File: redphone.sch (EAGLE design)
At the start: 228 parts, among them IC1 EP4CE22U14I7N, IC10 MPU9250, IC11 PCA9633TK, IC12 BME280, IC13 W25Q64FV, IC14 MC-1010-G, IC15 MAX2659, IC16 MP34DT01, IC17 APDS-9960, IC2 STM32F429NI, IC3 MT48LC16M16A2B4, IC4 MT48LC16M16A2B4, IC5 W25Q64FV, IC6 SIM800H, IC7 TPS65217, IC8 ESP8266, IC9 WM8903, M1 VIBRO, Q1 IRLML2502, Q2 IRLML2502, Q3 IRLML2502, Q4 IRLML2502, X1 USB, X2 OV5647, X3 RM68120_LCD, X4 MICRO_SIM_SDS8, X5 LG_P715_TS, X7 AUDIO-JACKSMD, Y1 2.4Ghz, Y3 2.4Ghz, Y4 GSM_PCB

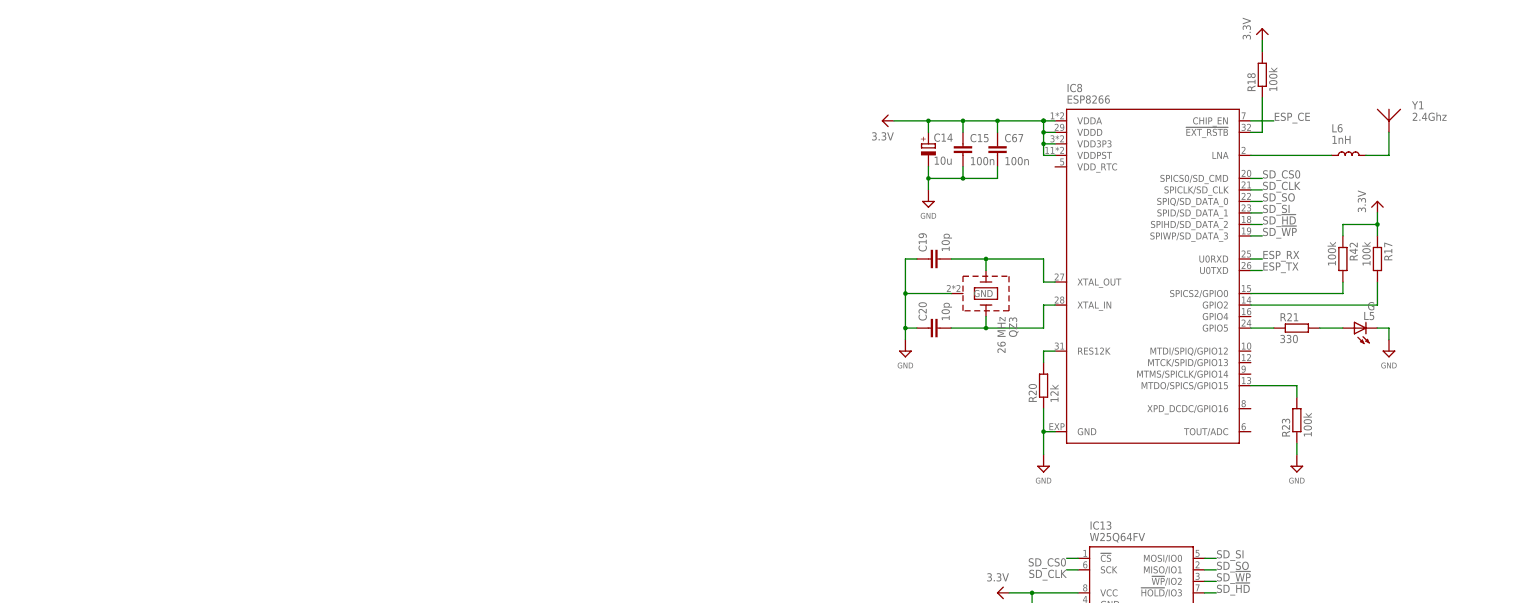
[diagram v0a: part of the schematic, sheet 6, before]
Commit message: esp8266 was replaced by esp32
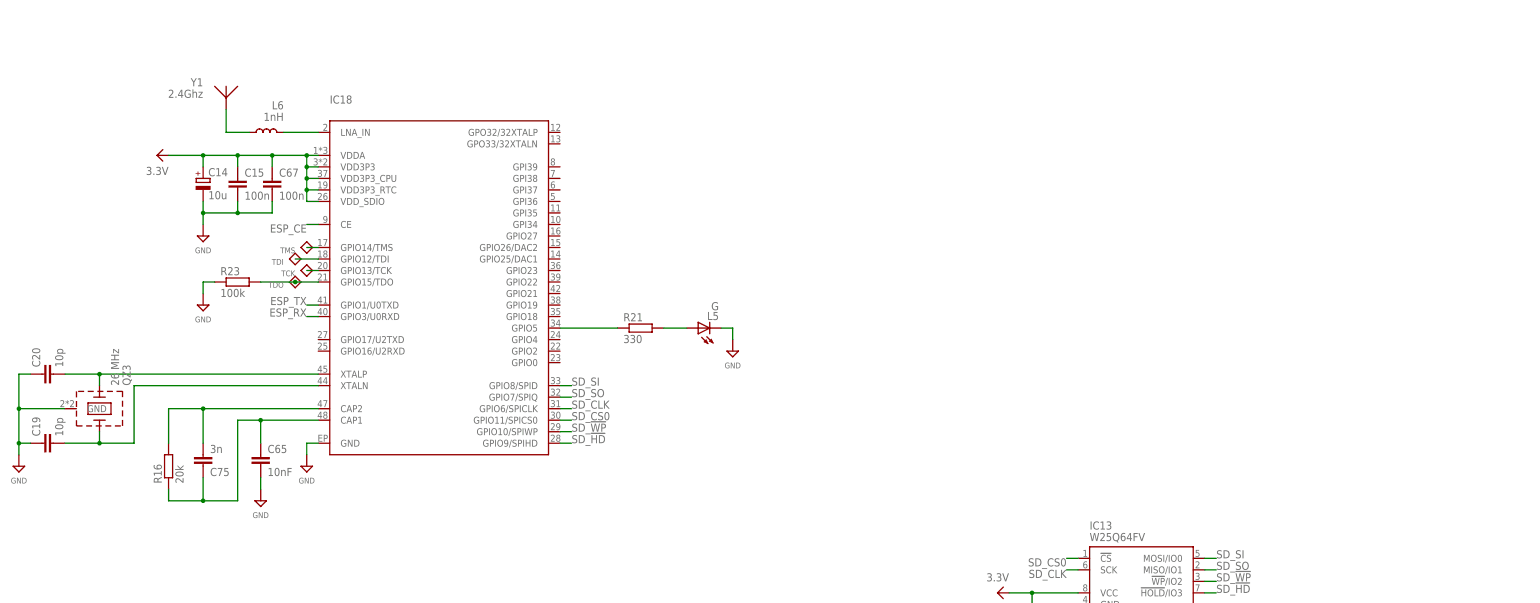
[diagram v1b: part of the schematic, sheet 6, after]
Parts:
- removed IC8: ESP8266, netcat:ESP8266
- removed R17, R18, R42: 100k, netcat:RESR0402
- removed R20: 12k, netcat:RESR0402
- added C65: 10nF, netcat:CAP0402
- added C75: 3n, netcat:CAP0402
- added IC18: (no value), netcat:ESP32
- added R16: 20k, netcat:RESR0402
- added TP_ESP_TCK: TCK, netcat:TP10R
- added TP_ESP_TDI: TDI, netcat:TP10R
- added TP_ESP_TDO: TDO, netcat:TP10R
- added TP_TMS: TMS, netcat:TP10R
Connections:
- removed net GPIO15: IC8.MTDO/SPICS/GPIO15, R23.2
- removed net N$103: IC8.GPIO5, R21.1
- removed net N$47: IC8.LNA, L6.P$1
- removed net N$71: IC8.SPICS2/GPIO0, R42.2
- removed net N$92: IC8.!EXT_RSTB, R18.1
- removed net N$94: IC8.GPIO2, R17.2
- new net N$25: IC18.LNA_IN, L6.P$1
- new net N$28: IC18.GPIO15/TDO, R23.2, TP_ESP_TDO.TEST
- new net N$30: C75.2, IC18.CAP2, R16.2
- new net N$31: IC18.GPIO14/TMS, TP_TMS.TEST
- new net N$32: IC18.GPIO12/TDI, TP_ESP_TDI.TEST
- new net N$33: IC18.GPIO13/TCK, TP_ESP_TCK.TEST
- new net N$34: IC18.GPIO5, R21.1
- net 3.3V: now also IC18.VDD3P3, IC18.VDD3P3_CPU, IC18.VDD3P3_RTC, IC18.VDDA, IC18.VDD_SDIO; no longer IC8.VDD3P3, IC8.VDDA, IC8.VDDD, IC8.VDDPST, R17.1, R18.2, R42.1
- net ESP_CE: now also IC18.CE; no longer IC8.CHIP_EN
- net ESP_RX: now also IC18.GPIO3/U0RXD; no longer IC8.U0RXD
- net ESP_TX: now also IC18.GPIO1/U0TXD; no longer IC8.U0TXD
- net GND: now also C65.2, IC18.GND; no longer IC8.GND, R20.1
- net N$24: now also C65.1, C75.1, IC18.CAP1, R16.1; no longer IC8.RES12K, R20.2
- net N$26: now also IC18.XTALN; no longer IC8.XTAL_OUT
- net N$27: now also IC18.XTALP; no longer IC8.XTAL_IN
- net SD_!HD!: now also IC18.GPIO9/SPIHD; no longer IC8.SPIHD/SD_DATA_2
- net SD_!WP!: now also IC18.GPIO10/SPIWP; no longer IC8.SPIWP/SD_DATA_3
- net SD_CLK: now also IC18.GPIO6/SPICLK; no longer IC8.SPICLK/SD_CLK
- net SD_CS0: now also IC18.GPIO11/SPICS0; no longer IC8.SPICS0/SD_CMD
- net SD_SI: now also IC18.GPIO8/SPID; no longer IC8.SPID/SD_DATA_1
- net SD_SO: now also IC18.GPIO7/SPIQ; no longer IC8.SPIQ/SD_DATA_0
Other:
- moved on the sheet: C14, C15, C19, C20, C67, L5, L6, QZ3, R21, R23, Y1
